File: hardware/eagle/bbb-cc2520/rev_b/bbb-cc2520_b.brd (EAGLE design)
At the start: 54.6 x 73.4 mm, 99 parts, among them J1 TC2030-IDC, P9/P8 BBB_HEADERS, U1 CC2520, U2 CC2520, U3 CAT24C256WI-GT3, U4 CC2591, U5 CD4051B-53B, U6 NRF51822QF, X1 NX2520SA, X2 NX2520SA, X3 16MHz

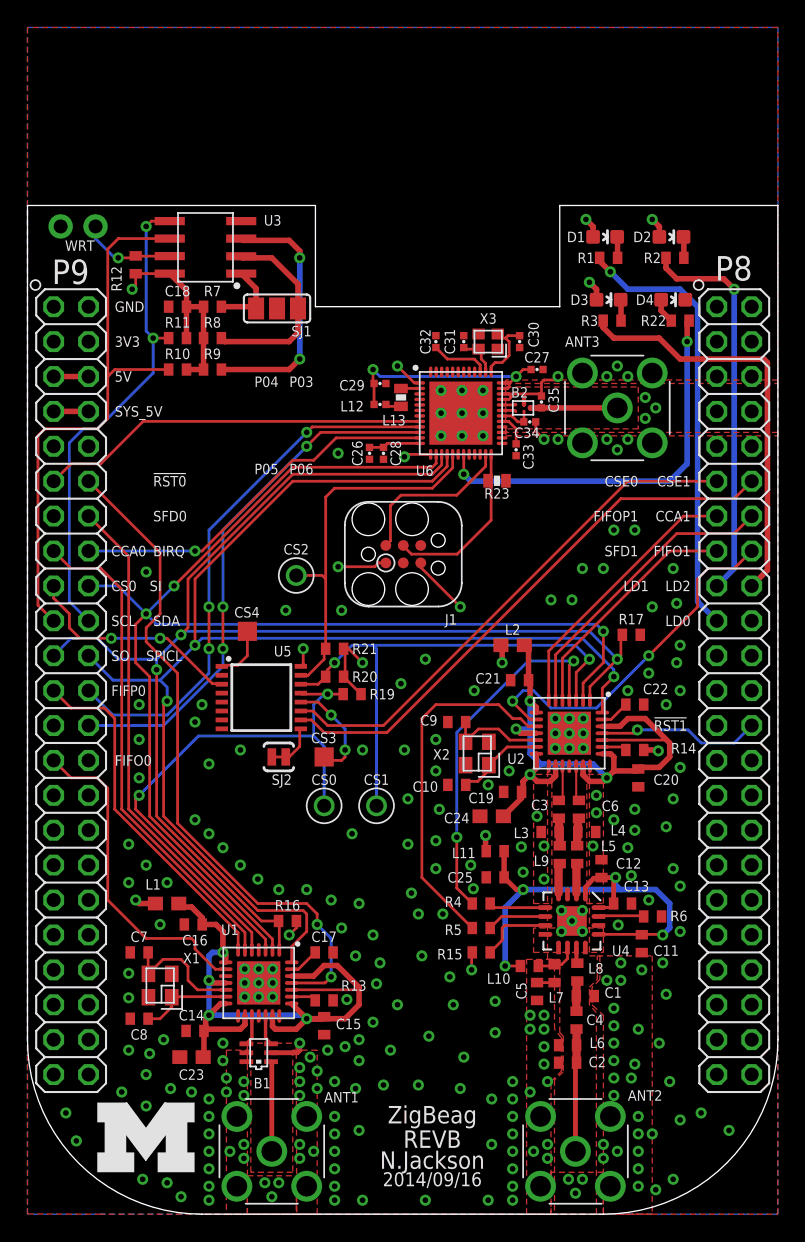
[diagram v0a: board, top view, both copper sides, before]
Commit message: cleaned up pcb
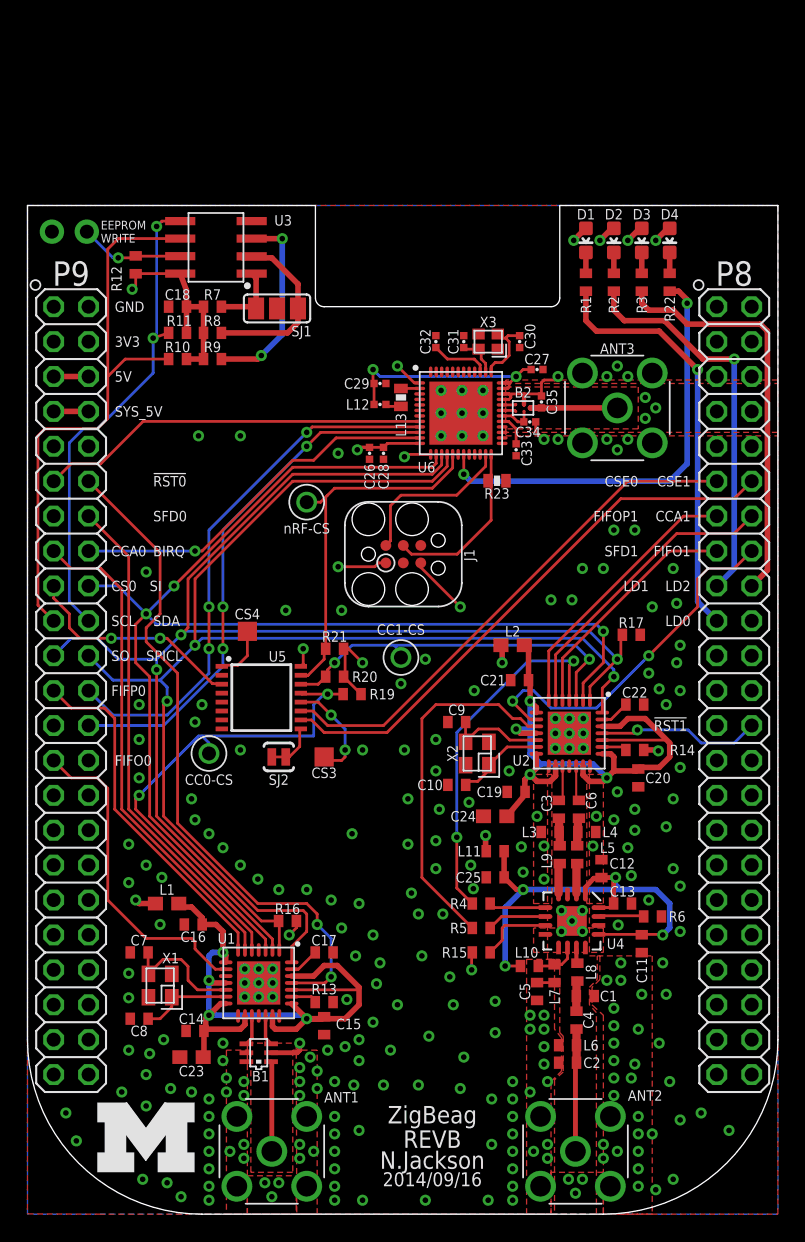
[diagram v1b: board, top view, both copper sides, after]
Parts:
- removed WRT: JUMPER-PTH-2-NO, SparkFun-Passives:PTH-JUMPER-2-NO_NO_SILK
- added J2: JUMPER-PTH-2-NO, SparkFun-Passives:PTH-JUMPER-2-NO_NO_SILK
- moved CS1 10.9 mm to (27.2, 40.5)
- moved CS0 9.21 mm to (13.2, 33.5)
- moved CS2 5.39 mm to (20.3, 51.8)
- moved D3 4.95 mm to (44.7, 70.9), turned to 180 degrees
- moved R2 4.79 mm to (42.7, 67.8), turned to 90 degrees
- moved D4 4.33 mm to (46.7, 70.9), turned to 180 degrees
- moved D2 4.20 mm to (42.7, 70.9), turned to 180 degrees
- moved R3 3.53 mm to (44.7, 67.8), turned to 90 degrees
- moved R22 2.90 mm to (46.7, 67.8), turned to 90 degrees
- moved R1 2.43 mm to (40.6, 67.8), turned to 90 degrees
- moved D1 1.42 mm to (40.6, 70.9), turned to 180 degrees
- moved U3 0.76 mm to (13.7, 70.4)
- moved R10 0.76 mm to (10.9, 62.2)
- moved R9 0.76 mm to (13.5, 62.2)
- moved R11 0.38 mm to (10.9, 64.1)
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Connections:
- net GND: now also J2.2; no longer D4.C, WRT.2
- net N$31: now also J2.1; no longer WRT.1
- net N$63: now also D4.C, R22.2; no longer D4.A, R22.1
- net N$64: now also R22.1; no longer R22.2
- net VCC: now also D4.A
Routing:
- net CS1: track 38.0 -> 27.3 mm
- net N$32: track 18.5 -> 14.4 mm
- net CS0: track 41.9 -> 38.0 mm
- net N$64: track 28.9 -> 31.9 mm
- net LED0: track 32.2 -> 30.6 mm
- net VCC: track 42.7 -> 43.8 mm, vias 12 -> 14
- net SCL: track 41.3 -> 42.4 mm
- net N$31: track 6.94 -> 7.65 mm
- net CS2: track 27.4 -> 26.7 mm
- net GND: vias 263 -> 265
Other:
- outline, holes or cut-outs redrawn
- board text added: "CC0-CS"
- board text added: "CC1-CS"
- board text added: "EEPROM WRITE"
- board text added: "nRF-CS"
- board text removed: "P03"
- board text removed: "P04"
- board text removed: "P05"
- board text removed: "P06"
